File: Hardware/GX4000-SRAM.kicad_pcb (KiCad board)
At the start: 2 copper layers, 7 parts, among them IC10 TMS4464, IC11 TMS4464, U1 IS62C1024AL-35QLI, U2 74HCT573, U3 74LVC1G32

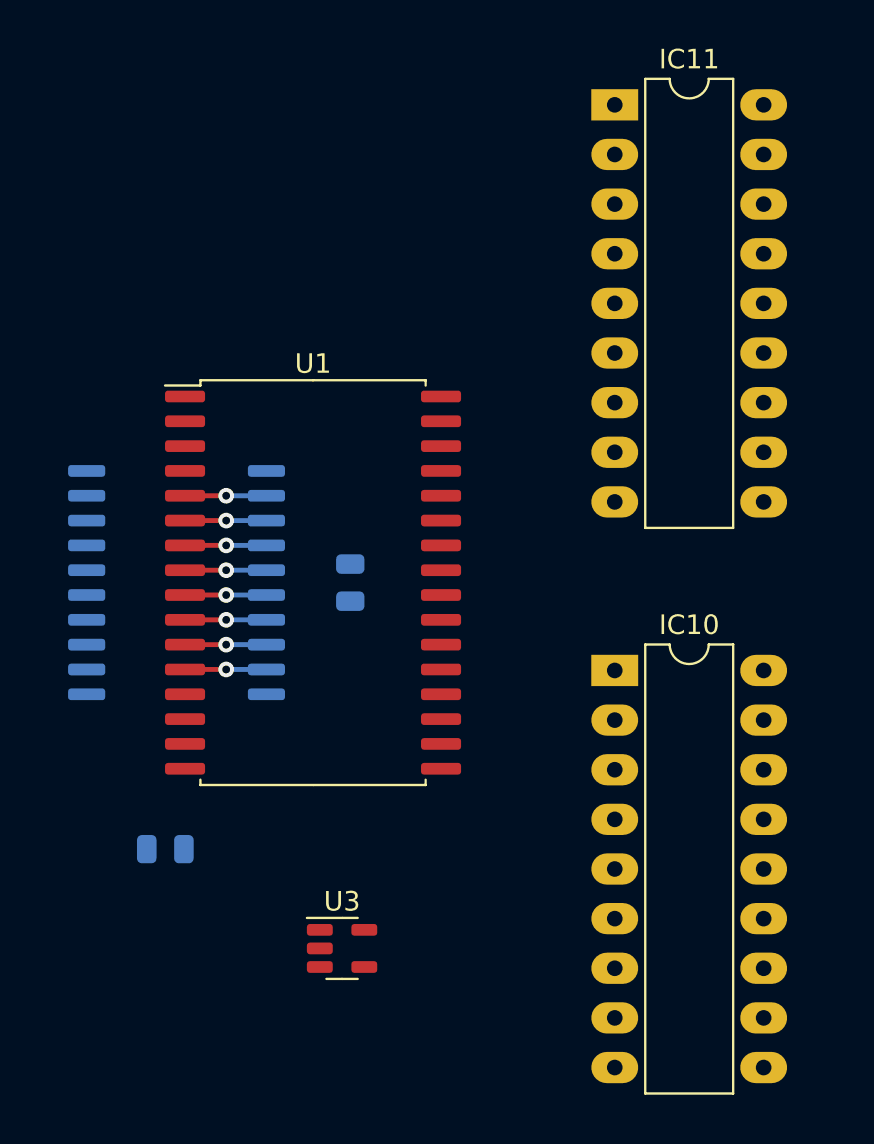
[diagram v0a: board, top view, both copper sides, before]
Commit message: Release PCB
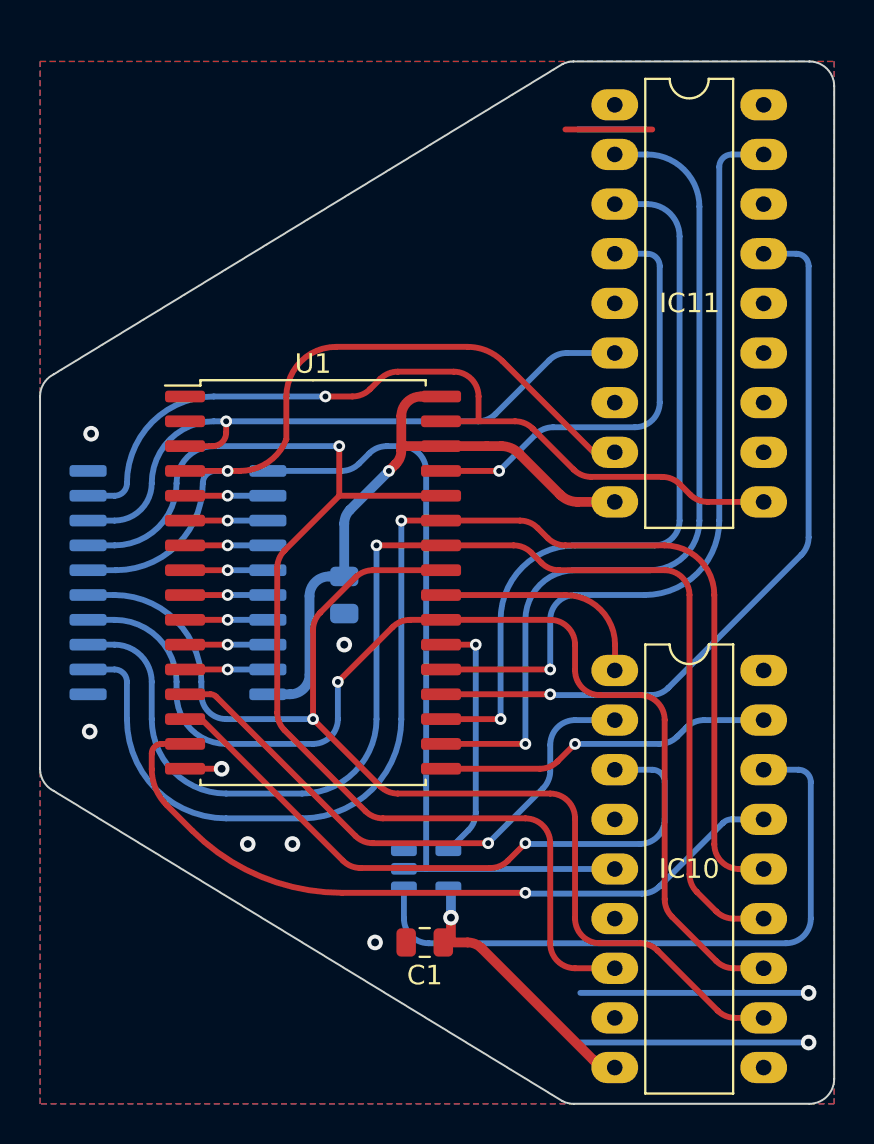
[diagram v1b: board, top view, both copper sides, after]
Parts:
- C1: moved to F.Cu
- U3: moved to B.Cu
- moved C1 14.1 mm to (141.4, 108.9)
- moved U3 5.93 mm to (141.5, 105.1)
- moved C2 0.71 mm to (137.3, 91.1)
- moved U2 0.07 mm to (128.8, 90.5)
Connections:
- IC10 pad 10: /MA7 -> unconnected-(IC10-Pad10)
- IC10 pad 15: /D6 -> /D2
- IC10 pad 17: /D7 -> /D3
- IC10 pad 2: /D4 -> /D0
- IC10 pad 3: /D5 -> /D1
- IC10 pad 4: /~{WE} -> unconnected-(IC10-Pad4)
- IC10 pad 6: /MA6 -> unconnected-(IC10-Pad6)
- IC10 pad 8: /MA4 -> unconnected-(IC10-Pad8)
- IC11 pad 10: unconnected-(IC11-Pad10) -> /MA7
- IC11 pad 15: /D2 -> /D6
- IC11 pad 17: /D3 -> /D7
- IC11 pad 2: /D0 -> /D4
- IC11 pad 3: /D1 -> /D5
- IC11 pad 4: unconnected-(IC11-Pad4) -> /~{WE}
- IC11 pad 6: unconnected-(IC11-Pad6) -> /MA6
- IC11 pad 8: unconnected-(IC11-Pad8) -> /MA4
- U3 pad 1: /~{RAS} -> /~{CAS}
- U3 pad 2: /~{CAS} -> /~{RAS}
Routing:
- net /MA0: track 0.00 -> 67.5 mm, vias 0 -> 1
- net /MA1: track 0.00 -> 66.9 mm, vias 0 -> 1
- net /MA5: track 0.00 -> 61.8 mm, vias 0 -> 1
- net /MA3: track 0.00 -> 60.2 mm, vias 0 -> 1
- net /MA2: track 0.00 -> 56.2 mm, vias 0 -> 1
- net VCC: track 0.00 -> 47.1 mm, vias 0 -> 2
- net /D4: track 0.00 -> 44.1 mm, vias 0 -> 1
- net /MA7: track 0.00 -> 43.0 mm, vias 0 -> 1
- net /~{RAS}: track 0.00 -> 40.4 mm
- net /D7: track 0.00 -> 40.2 mm, vias 0 -> 1
- net /D6: track 0.00 -> 38.9 mm, vias 0 -> 1
- net /D5: track 0.00 -> 38.7 mm, vias 0 -> 1
- net /D2: track 0.00 -> 38.2 mm, vias 0 -> 1
- net /MA4: track 0.00 -> 38.1 mm, vias 0 -> 1
- net /MA6: track 0.00 -> 34.0 mm, vias 0 -> 1
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- added copper zone on B.Cu, net GND
- added copper zone on F.Cu, net GND
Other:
- board outline added: 40.6 x 53.3 mm
